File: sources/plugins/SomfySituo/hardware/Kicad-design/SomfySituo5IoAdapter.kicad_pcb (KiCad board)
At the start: 2 copper layers, 25.4 x 21.8 mm, 30 parts, among them J1 USB_OTG, J10 Conn_01x01, J11 Conn_01x01, J12 Conn_01x01, J13 Conn_01x01, J15 ICSP, J2 Conn_01x01, J3 Conn_01x01, J4 Conn_01x01, J5 Conn_01x01, J6 Conn_01x01, J7 Conn_01x01, J8 Conn_01x01, J9 Conn_01x01, U1 FT230X, U2 PIC16F688

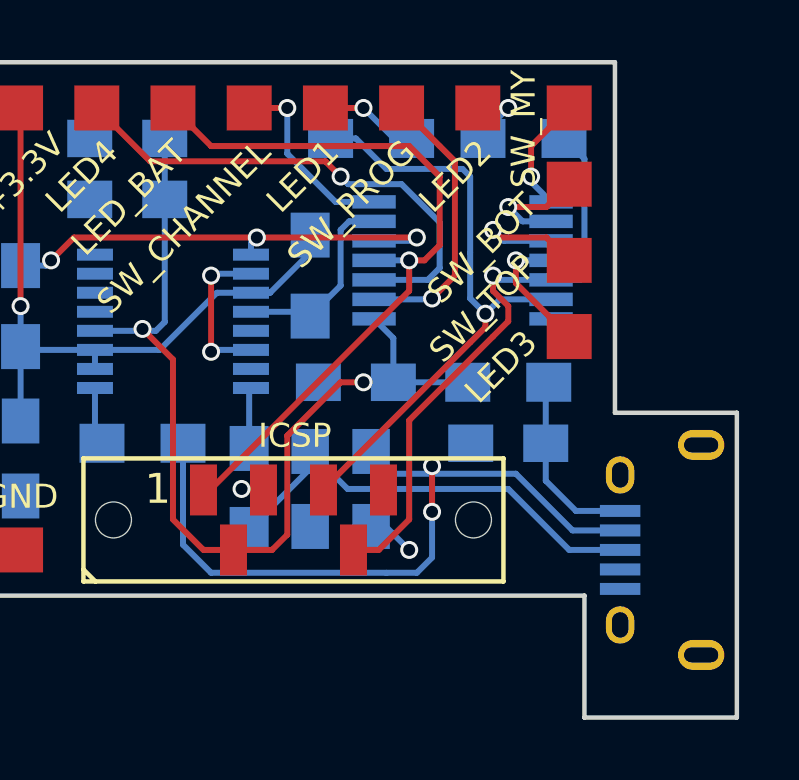
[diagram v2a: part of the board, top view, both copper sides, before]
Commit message: Mov USB connector
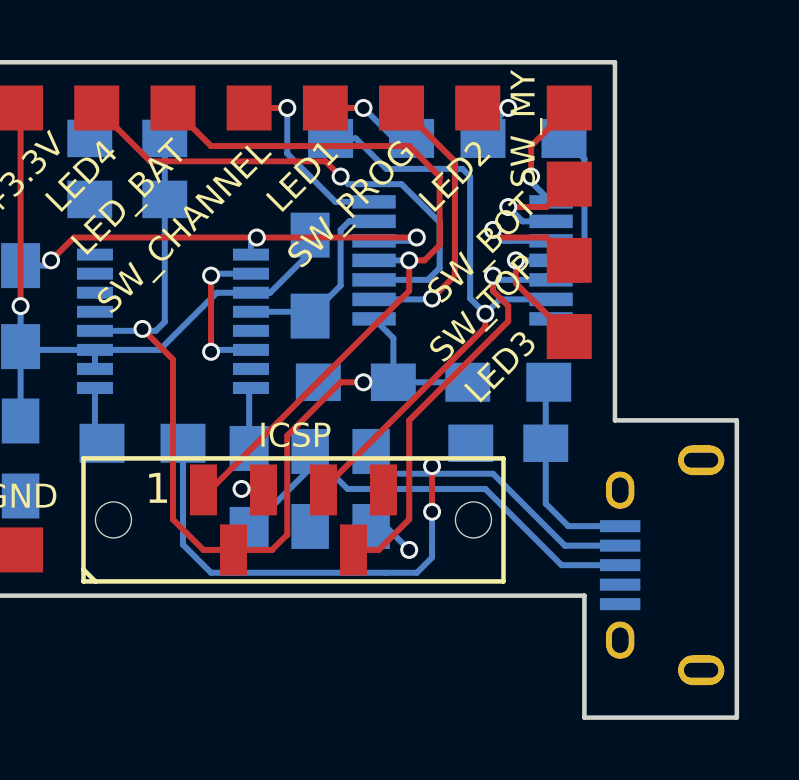
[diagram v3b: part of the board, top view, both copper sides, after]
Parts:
- moved J1 0.51 mm to (131.1, 127.0)
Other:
- outline, holes or cut-outs redrawn
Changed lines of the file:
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@@
   (page A4)
   (layers
-    (0 F.Cu signal hide)
-    (31 B.Cu signal hide)
+    (0 F.Cu signal)
+    (31 B.Cu signal)
     (32 B.Adhes user)
     (33 F.Adhes user)
@@
   )
   (module Connectors:USB_Micro-B (layer B.Cu)
-    (at 131.064 126.492 270)
+    (at 131.064 127 270)
     (descr "Micro USB Type B Receptacle")
     (tags "USB USB_B USB_micro USB_OTG")
@@
       (net 2 GND))
   )
+  (dimension 11.938 (width 0.3) (layer Cmts.User)
+    (gr_text "11,938 mm" (at 139.446 115.316 90) (layer Cmts.User)
+      (effects (font (size 1.5 1.5) (thickness 0.3)))
+    )
+    (feature1 (pts (xy 133.604 110.236) (xy 140.368 110.236)))
+    (feature2 (pts (xy 133.604 122.174) (xy 140.368 122.174)))
+    (crossbar (pts (xy 137.668 122.174) (xy 137.668 110.236)))
+    (arrow1a (pts (xy 137.668 110.236) (xy 138.254421 111.362504)))
+    (arrow1b (pts (xy 137.668 110.236) (xy 137.081579 111.362504)))
+    (arrow2a (pts (xy 137.668 122.174) (xy 138.254421 121.047496)))
+    (arrow2b (pts (xy 137.668 122.174) (xy 137.081579 121.047496)))
+  )
+  (dimension 9.906 (width 0.3) (layer Cmts.User)
+    (gr_text "9,906 mm" (at 140.97 126.238 90) (layer Cmts.User)
+      (effects (font (size 1.5 1.5) (thickness 0.3)))
+    )
+    (feature1 (pts (xy 133.604 122.174) (xy 140.368 122.174)))
+    (feature2 (pts (xy 133.604 132.08) (xy 140.368 132.08)))
+    (crossbar (pts (xy 137.668 132.08) (xy 137.668 122.174)))
+    (arrow1a (pts (xy 137.668 122.174) (xy 138.254421 123.300504)))
+    (arrow1b (pts (xy 137.668 122.174) (xy 137.081579 123.300504)))
+    (arrow2a (pts (xy 137.668 132.08) (xy 138.254421 130.953496)))
+    (arrow2b (pts (xy 137.668 132.08) (xy 137.081579 130.953496)))
+  )
+  (gr_line (start 133.604 122.174) (end 133.604 132.08) (angle 90) (layer Edge.Cuts) (width 0.15))
+  (gr_line (start 129.54 122.174) (end 129.54 110.236) (angle 90) (layer Edge.Cuts) (width 0.15))
+  (gr_line (start 133.604 122.174) (end 129.54 122.174) (angle 90) (layer Edge.Cuts) (width 0.15))
   (gr_text LED3 (at 126.746 119.38 45) (layer F.SilkS)
     (effects (font (size 0.8 0.8) (thickness 0.15)) (justify right))
@@
     (arrow2b (pts (xy 145.288 132.08) (xy 144.701579 130.953496)))
   )
-  (dimension 10.16 (width 0.3) (layer Cmts.User)
-    (gr_text "10,160 mm" (at 139.7 130.048 270) (layer Cmts.User)
-      (effects (font (size 1.5 1.5) (thickness 0.3)))
-    )
-    (feature1 (pts (xy 133.604 132.08) (xy 140.368 132.08)))
-    (feature2 (pts (xy 133.604 121.92) (xy 140.368 121.92)))
-    (crossbar (pts (xy 137.668 121.92) (xy 137.668 132.08)))
-    (arrow1a (pts (xy 137.668 132.08) (xy 137.081579 130.953496)))
-    (arrow1b (pts (xy 137.668 132.08) (xy 138.254421 130.953496)))
-    (arrow2a (pts (xy 137.668 121.92) (xy 137.081579 123.046504)))
-    (arrow2b (pts (xy 137.668 121.92) (xy 138.254421 123.046504)))
-  )
-  (dimension 11.684 (width 0.3) (layer Cmts.User)
-    (gr_text "11,684 mm" (at 141.224 113.792 90) (layer Cmts.User)
-      (effects (font (size 1.5 1.5) (thickness 0.3)))
-    )
-    (feature1 (pts (xy 133.604 110.236) (xy 140.368 110.236)))
-    (feature2 (pts (xy 133.604 121.92) (xy 140.368 121.92)))
-    (crossbar (pts (xy 137.668 121.92) (xy 137.668 110.236)))
-    (arrow1a (pts (xy 137.668 110.236) (xy 138.254421 111.362504)))
-    (arrow1b (pts (xy 137.668 110.236) (xy 137.081579 111.362504)))
-    (arrow2a (pts (xy 137.668 121.92) (xy 138.254421 120.793496)))
-    (arrow2b (pts (xy 137.668 121.92) (xy 137.081579 120.793496)))
-  )
   (dimension 4.064 (width 0.3) (layer Cmts.User)
     (gr_text "4,064 mm" (at 133.096 102.616) (layer Cmts.User)
@@
     (effects (font (size 1 1) (thickness 0.2)))
   )
-  (gr_line (start 129.54 110.236) (end 129.54 121.92) (angle 90) (layer Edge.Cuts) (width 0.15))
   (gr_line (start 128.524 132.08) (end 128.524 128.016) (angle 90) (layer Edge.Cuts) (width 0.15))
-  (gr_line (start 133.604 121.92) (end 129.54 121.92) (angle 90) (layer Edge.Cuts) (width 0.15))
-  (gr_line (start 133.604 132.08) (end 133.604 121.92) (angle 90) (layer Edge.Cuts) (width 0.15))
   (gr_line (start 133.604 132.08) (end 128.524 132.08) (angle 90) (layer Edge.Cuts) (width 0.15))
   (segment (start 116.824 126.492) (end 115.824 126.492) (width 0.2) (layer F.Cu) (net 1))
@@
   (segment (start 121.9 125.71) (end 122.682 126.492) (width 0.2) (layer B.Cu) (net 2))
   (via (at 122.682 126.492) (size 0.6) (drill 0.4) (layers F.Cu B.Cu) (net 2))
+  (segment (start 120.63 124.46) (end 125.222 124.46) (width 0.2) (layer B.Cu) (net 3))
+  (segment (start 119.38 123.21) (end 120.63 124.46) (width 0.2) (layer B.Cu) (net 3))
+  (segment (start 127.762 127) (end 129.714 127) (width 0.2) (layer B.Cu) (net 3) (status 800000))
+  (segment (start 125.222 124.46) (end 127.762 127) (width 0.2) (layer B.Cu) (net 3))
   (segment (start 117.348 125.81) (end 119.38 123.778) (width 0.2) (layer B.Cu) (net 3))
   (segment (start 119.38 123.778) (end 119.38 123.21) (width 0.2) (layer B.Cu) (net 3))
-  (segment (start 129.714 126.492) (end 128.016 126.492) (width 0.2) (layer B.Cu) (net 3))
-  (segment (start 120.63 124.46) (end 119.38 123.21) (width 0.2) (layer B.Cu) (net 3))
-  (segment (start 125.984 124.46) (end 120.63 124.46) (width 0.2) (layer B.Cu) (net 3))
-  (segment (start 128.016 126.492) (end 125.984 124.46) (width 0.2) (layer B.Cu) (net 3))
-  (segment (start 123.444 125.222) (end 123.444 126.746) (width 0.2) (layer B.Cu) (net 4))
+  (via (at 123.444 123.698) (size 0.6) (drill 0.4) (layers F.Cu B.Cu) (net 4))
+  (segment (start 123.444 126.746) (end 122.936 127.254) (width 0.2) (layer B.Cu) (net 4))
+  (segment (start 122.936 127.254) (end 121.92 127.254) (width 0.2) (layer B.Cu) (net 4))
+  (segment (start 115.142 122.936) (end 115.142 126.318) (width 0.2) (layer B.Cu) (net 4))
+  (segment (start 123.444 125.222) (end 123.444 123.698) (width 0.2) (layer F.Cu) (net 4))
+  (via (at 123.444 125.222) (size 0.6) (drill 0.4) (layers F.Cu B.Cu) (net 4))
+  (segment (start 116.078 127.254) (end 121.92 127.254) (width 0.2) (layer B.Cu) (net 4))
   (segment (start 115.142 126.318) (end 116.078 127.254) (width 0.2) (layer B.Cu) (net 4))
-  (segment (start 116.078 127.254) (end 121.92 127.254) (width 0.2) (layer B.Cu) (net 4))
-  (via (at 123.444 125.222) (size 0.6) (drill 0.4) (layers F.Cu B.Cu) (net 4))
-  (segment (start 123.444 125.222) (end 123.444 123.698) (width 0.2) (layer F.Cu) (net 4))
-  (via (at 123.444 123.698) (size 0.6) (drill 0.4) (layers F.Cu B.Cu) (net 4))
-  (segment (start 123.444 123.952) (end 123.444 123.698) (width 0.2) (layer B.Cu) (net 4))
-  (segment (start 115.142 126.318) (end 115.142 122.936) (width 0.2) (layer B.Cu) (net 4))
-  (segment (start 122.936 127.254) (end 121.92 127.254) (width 0.2) (layer B.Cu) (net 4))
-  (segment (start 123.444 126.746) (end 122.936 127.254) (width 0.2) (layer B.Cu) (net 4))
-  (segment (start 129.714 125.842) (end 128.128 125.842) (width 0.2) (layer B.Cu) (net 4))
+  (segment (start 123.444 126.492) (end 123.444 126.746) (width 0.2) (layer B.Cu) (net 4))
+  (segment (start 123.444 125.222) (end 123.444 126.492) (width 0.2) (layer B.Cu) (net 4))
+  (segment (start 123.444 123.698) (end 123.444 123.952) (width 0.2) (layer B.Cu) (net 4))
+  (segment (start 129.714 126.35) (end 127.874 126.35) (width 0.2) (layer B.Cu) (net 4) (status 400000))
   (segment (start 122.154 123.952) (end 121.412 123.21) (width 0.2) (layer B.Cu) (net 4))
-  (segment (start 126.238 123.952) (end 123.444 123.952) (width 0.2) (layer B.Cu) (net 4))
+  (segment (start 125.476 123.952) (end 123.444 123.952) (width 0.2) (layer B.Cu) (net 4))
   (segment (start 123.444 123.952) (end 122.154 123.952) (width 0.2) (layer B.Cu) (net 4))
-  (segment (start 128.128 125.842) (end 126.238 123.952) (width 0.2) (layer B.Cu) (net 4))
+  (segment (start 127.874 126.35) (end 125.476 123.952) (width 0.2) (layer B.Cu) (net 4))
   (segment (start 112.208 120.4595) (end 112.208 119.8245) (width 0.2) (layer B.Cu) (net 5))
   (segment (start 109.728 119.714) (end 109.728 118.364) (width 0.2) (layer B.Cu) (net 5))
@@
   (via (at 116.078 117.348) (size 0.6) (drill 0.4) (layers F.Cu B.Cu) (net 22))
   (segment (start 116.1415 117.2845) (end 116.078 117.348) (width 0.2) (layer B.Cu) (net 22))
-  (segment (start 127.234 122.936) (end 127.234 124.186) (width 0.2) (layer B.Cu) (net 23))
-  (segment (start 128.24 125.192) (end 129.714 125.192) (width 0.2) (layer B.Cu) (net 23))
-  (segment (start 127.234 124.186) (end 128.24 125.192) (width 0.2) (layer B.Cu) (net 23))
+  (segment (start 129.714 125.7) (end 127.986 125.7) (width 0.2) (layer B.Cu) (net 23) (status 400000))
+  (segment (start 127.234 124.948) (end 127.234 122.936) (width 0.2) (layer B.Cu) (net 23) (status 800000))
+  (segment (start 127.986 125.7) (end 127.234 124.948) (width 0.2) (layer B.Cu) (net 23))
   (segment (start 127.234 122.936) (end 127.234 121.004) (width 0.2) (layer B.Cu) (net 23))
   (segment (start 127.234 121.004) (end 127.334 120.904) (width 0.2) (layer B.Cu) (net 23))
-  (segment (start 129.714 125.192) (end 129.256 125.192) (width 0.2) (layer B.Cu) (net 23))
   (segment (start 127.234 123.17) (end 127.234 122.936) (width 0.2) (layer B.Cu) (net 23))
   (zone (net 2) (net_name GND) (layer B.Cu) (hatch edge 0.508)
@@
     (polygon
       (pts
-        (xy 108.204 110.236) (xy 129.54 110.236) (xy 129.54 121.92) (xy 133.604 121.92) (xy 133.604 132.08)
+        (xy 108.204 110.236) (xy 129.54 110.236) (xy 129.54 122.174) (xy 133.604 122.174) (xy 133.604 132.08)
         (xy 128.524 132.08) (xy 128.524 128.016) (xy 108.204 128.016)
       )
@@
     (polygon
       (pts
-        (xy 108.204 110.236) (xy 129.54 110.236) (xy 129.54 121.92) (xy 133.604 121.92) (xy 133.604 132.08)
+        (xy 108.204 110.236) (xy 129.54 110.236) (xy 129.54 122.174) (xy 133.604 122.174) (xy 133.604 132.08)
         (xy 128.524 132.08) (xy 128.524 128.016) (xy 108.204 128.016)
       )
